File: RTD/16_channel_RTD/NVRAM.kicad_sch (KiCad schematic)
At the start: 2 parts, among them U8 MB85RS64

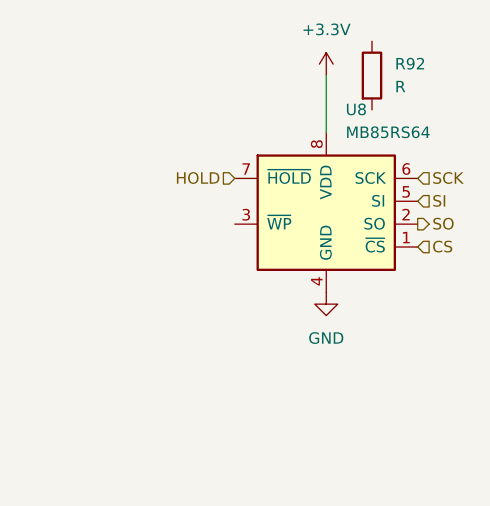
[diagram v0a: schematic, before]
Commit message: ERC free
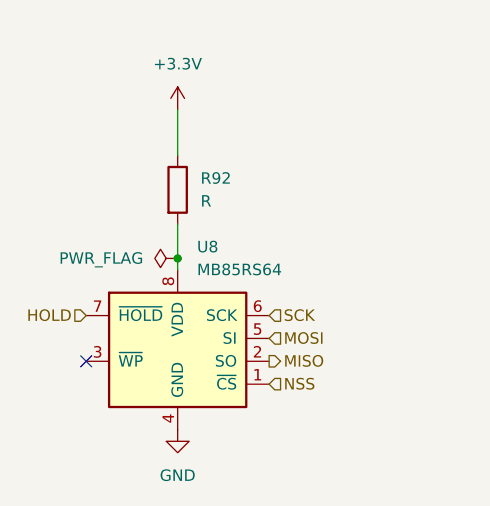
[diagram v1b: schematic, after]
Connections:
- net +3.3V: now also R92.1; no longer U8.8 (VDD)
- net at R92.2: now also U8.8 (VDD)
- net CS renamed NSS
- net SI renamed MOSI
- net SO renamed MISO
- no-connect marks 0 -> 1
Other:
- moved on the sheet: R92, U8
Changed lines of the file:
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@@
 	(generator_version "9.0")
 	(paper "A4")
+	(junction
+		(at 83.82 72.39)
+		(diameter 0)
+		(color 0 0 0 0)
+	)
+	(no_connect
+		(at 73.66 83.82)
+	)
 	(wire
 		(pts
-			(xy 100.33 52.07) (xy 100.33 58.42)
+			(xy 83.82 55.88) (xy 83.82 60.96)
 		)
 		(stroke
@@
 		)
 	)
-	(hierarchical_label "SI"
+	(wire
+		(pts
+			(xy 83.82 68.58) (xy 83.82 72.39)
+		)
+		(stroke
+			(width 0)
+			(type default)
+		)
+	)
+	(wire
+		(pts
+			(xy 83.82 72.39) (xy 83.82 73.66)
+		)
+		(stroke
+			(width 0)
+			(type default)
+		)
+	)
+	(hierarchical_label "MOSI"
 		(shape input)
-		(at 110.49 66.04 0)
+		(at 93.98 81.28 0)
 		(effects
 			(font
@@
 		)
 	)
-	(hierarchical_label "CS"
+	(hierarchical_label "NSS"
 		(shape input)
-		(at 110.49 71.12 0)
+		(at 93.98 86.36 0)
 		(effects
 			(font
@@
 	(hierarchical_label "SCK"
 		(shape input)
-		(at 110.49 63.5 0)
+		(at 93.98 78.74 0)
 		(effects
 			(font
@@
 	(hierarchical_label "HOLD"
 		(shape input)
-		(at 90.17 63.5 180)
+		(at 73.66 78.74 180)
 		(effects
 			(font
@@
 		)
 	)
-	(hierarchical_label "SO"
+	(hierarchical_label "MISO"
 		(shape output)
-		(at 110.49 68.58 0)
+		(at 93.98 83.82 0)
 		(effects
 			(font
@@
 	(symbol
 		(lib_id "power:+3.3V")
-		(at 100.33 52.07 0)
+		(at 83.82 55.88 0)
 		(unit 1)
 		(exclude_from_sim no)
@@
 		(fields_autoplaced yes)
 		(property "Reference" "#PWR061"
-			(at 100.33 55.88 0)
+			(at 83.82 59.69 0)
 			(effects
 				(font
@@
 		)
 		(property "Value" "+3.3V"
-			(at 100.33 46.99 0)
+			(at 83.82 50.8 0)
 			(effects
 				(font
@@
 		)
 		(property "Footprint" ""
-			(at 100.33 52.07 0)
+			(at 83.82 55.88 0)
 			(effects
 				(font
@@
 		)
 		(property "Datasheet" ""
-			(at 100.33 52.07 0)
+			(at 83.82 55.88 0)
 			(effects
 				(font
@@
 		)
 		(property "Description" "Power symbol creates a global label with name \"+3.3V\""
-			(at 100.33 52.07 0)
+			(at 83.82 55.88 0)
 			(effects
 				(font
@@
 	(symbol
 		(lib_id "power:GND")
-		(at 100.33 76.2 0)
+		(at 83.82 91.44 0)
 		(unit 1)
 		(exclude_from_sim no)
@@
 		(fields_autoplaced yes)
 		(property "Reference" "#PWR060"
-			(at 100.33 82.55 0)
+			(at 83.82 97.79 0)
 			(effects
 				(font
@@
 		)
 		(property "Value" "GND"
-			(at 100.33 81.28 0)
+			(at 83.82 96.52 0)
 			(effects
 				(font
@@
 		)
 		(property "Footprint" ""
-			(at 100.33 76.2 0)
+			(at 83.82 91.44 0)
 			(effects
 				(font
@@
 		)
 		(property "Datasheet" ""
-			(at 100.33 76.2 0)
+			(at 83.82 91.44 0)
 			(effects
 				(font
@@
 		)
 		(property "Description" "Power symbol creates a global label with name \"GND\" , ground"
-			(at 100.33 76.2 0)
+			(at 83.82 91.44 0)
 			(effects
 				(font
@@
 	(symbol
 		(lib_id "Memory_NVRAM:MB85RS64")
-		(at 100.33 66.04 0)
+		(at 83.82 81.28 0)
 		(unit 1)
 		(exclude_from_sim no)
@@
 		(fields_autoplaced yes)
 		(property "Reference" "U8"
-			(at 102.4733 55.88 0)
+			(at 85.9633 71.12 0)
 			(effects
 				(font
@@
 		)
 		(property "Value" "MB85RS64"
-			(at 102.4733 58.42 0)
+			(at 85.9633 73.66 0)
 			(effects
 				(font
@@
 		)
 		(property "Footprint" ""
-			(at 91.44 67.31 0)
+			(at 74.93 82.55 0)
 			(effects
 				(font
@@
 		)
 		(property "Datasheet" "http://www.fujitsu.com/downloads/MICRO/fme/fram/datasheet-MB85RS64.pdf"
-			(at 91.44 67.31 0)
+			(at 74.93 82.55 0)
 			(effects
 				(font
@@
 		)
 		(property "Description" "FRAM memory with SPI interface, SOIC-8 SON-8"
-			(at 100.33 66.04 0)
+			(at 83.82 81.28 0)
 			(effects
 				(font
@@
 	(symbol
 		(lib_id "Device:R")
-		(at 105.41 52.07 0)
+		(at 83.82 64.77 0)
 		(unit 1)
 		(exclude_from_sim no)
@@
 		(fields_autoplaced yes)
 		(property "Reference" "R92"
-			(at 107.95 50.7999 0)
+			(at 86.36 63.4999 0)
 			(effects
 				(font
@@
 		)
 		(property "Value" "R"
-			(at 107.95 53.3399 0)
+			(at 86.36 66.0399 0)
 			(effects
 				(font
@@
 		)
 		(property "Footprint" ""
-			(at 103.632 52.07 90)
+			(at 82.042 64.77 90)
 			(effects
 				(font
@@
 		)
 		(property "Datasheet" "~"
-			(at 105.41 52.07 0)
+			(at 83.82 64.77 0)
 			(effects
 				(font
@@
 		)
 		(property "Description" "Resistor"
-			(at 105.41 52.07 0)
+			(at 83.82 64.77 0)
 			(effects
 				(font
@@
 					(unit 1)
 				)
+			)
+		)
+	)
+	(symbol
+		(lib_id "power:PWR_FLAG")
+		(at 83.82 72.39 90)
+		(unit 1)
+		(exclude_from_sim no)
+		(in_bom yes)
+		(on_board yes)
+		(dnp no)
+		(fields_autoplaced yes)
+		(property "Reference" "#FLG06"
+			(at 81.915 72.39 0)
+			(effects
+				(font
+					(size 1.27 1.27)
+				)
+				(hide yes)
+			)
+		)
+		(property "Value" "PWR_FLAG"
+			(at 80.01 72.3899 90)
+			(effects
+				(font
+					(size 1.27 1.27)
+				)
+				(justify left)
+			)
+		)
+		(property "Footprint" ""
+			(at 83.82 72.39 0)
+			(effects
+				(font
+					(size 1.27 1.27)
+				)
+				(hide yes)
+			)
+		)
+		(property "Datasheet" "~"
+			(at 83.82 72.39 0)
+			(effects
+				(font
+					(size 1.27 1.27)
+				)
+				(hide yes)
+			)
+		)
+		(property "Description" "Special symbol for telling ERC where power comes from"
+			(at 83.82 72.39 0)
+			(effects
+				(font
+					(size 1.27 1.27)
+				)
+				(hide yes)
+			)
+		)
+		(pin "1"
+		)
+		(instances
+			(project "16_channel_RTD"
+				(path "/7efa64d7-6b48-4f49-bdce-9f524c18a79f/42c94546-e431-4e8e-b95c-11e84c33e808"
+					(reference "#FLG06")
+					(unit 1)
+				)
